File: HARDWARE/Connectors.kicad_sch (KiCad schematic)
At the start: 11 parts, among them J12 Conn_02x08_Odd_Even, J13 Conn_02x10_Odd_Even, J14 Conn_02x15_Odd_Even, J15 Conn_02x17_Odd_Even, J16 Conn_02x36_Odd_Even, J17 Conn_02x36_Odd_Even

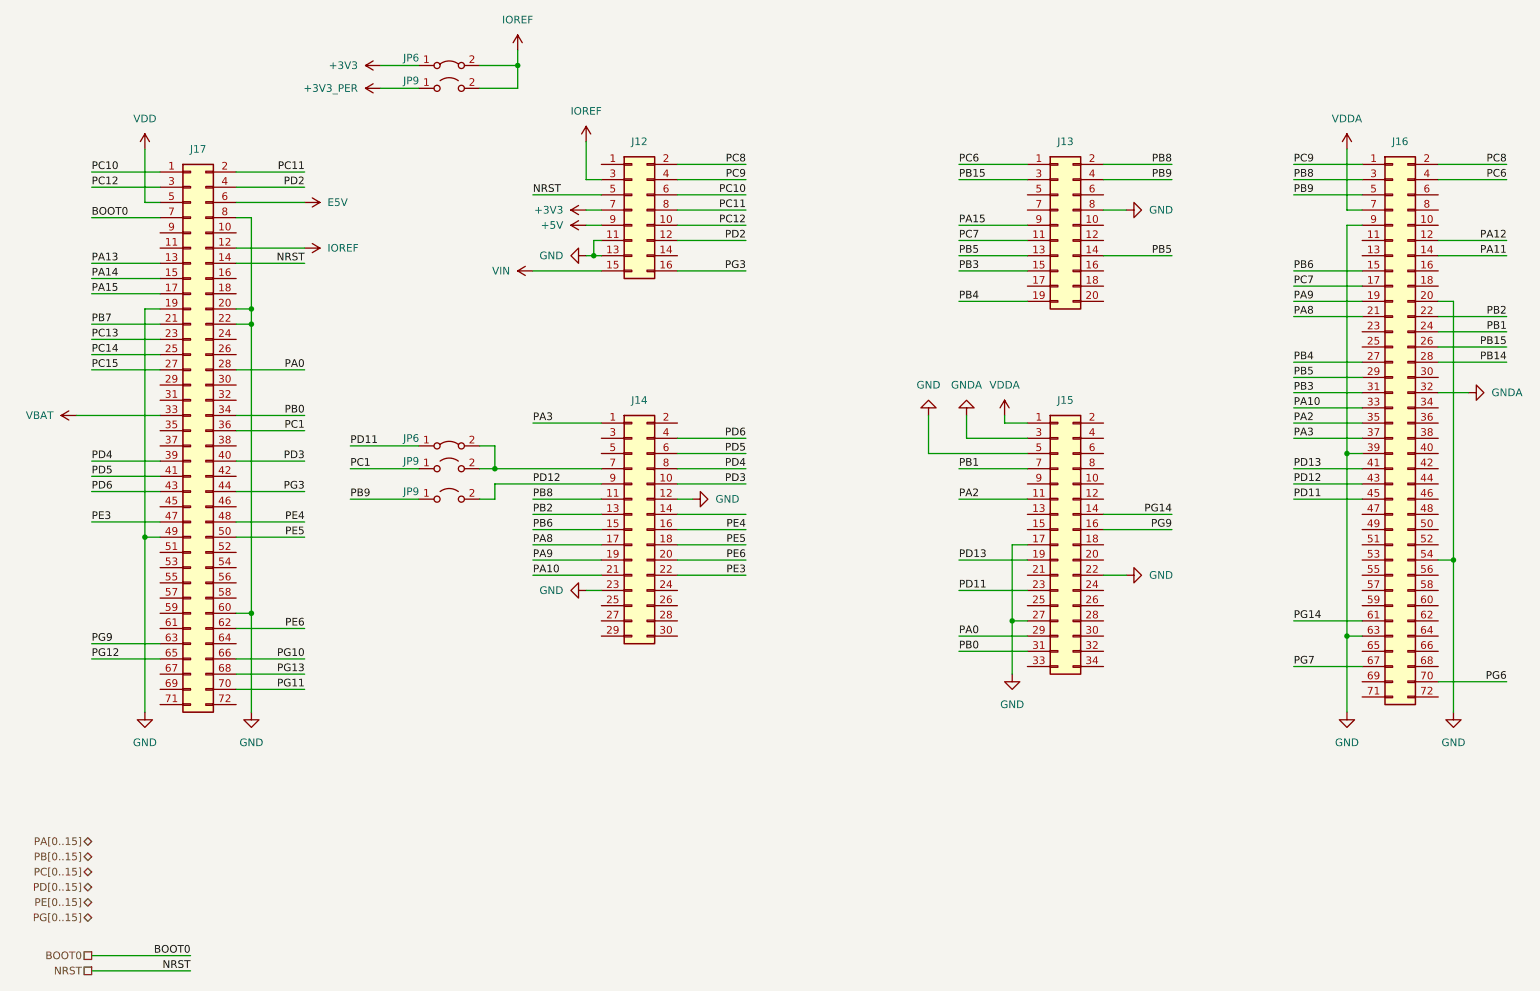
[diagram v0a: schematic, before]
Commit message: schematic capture
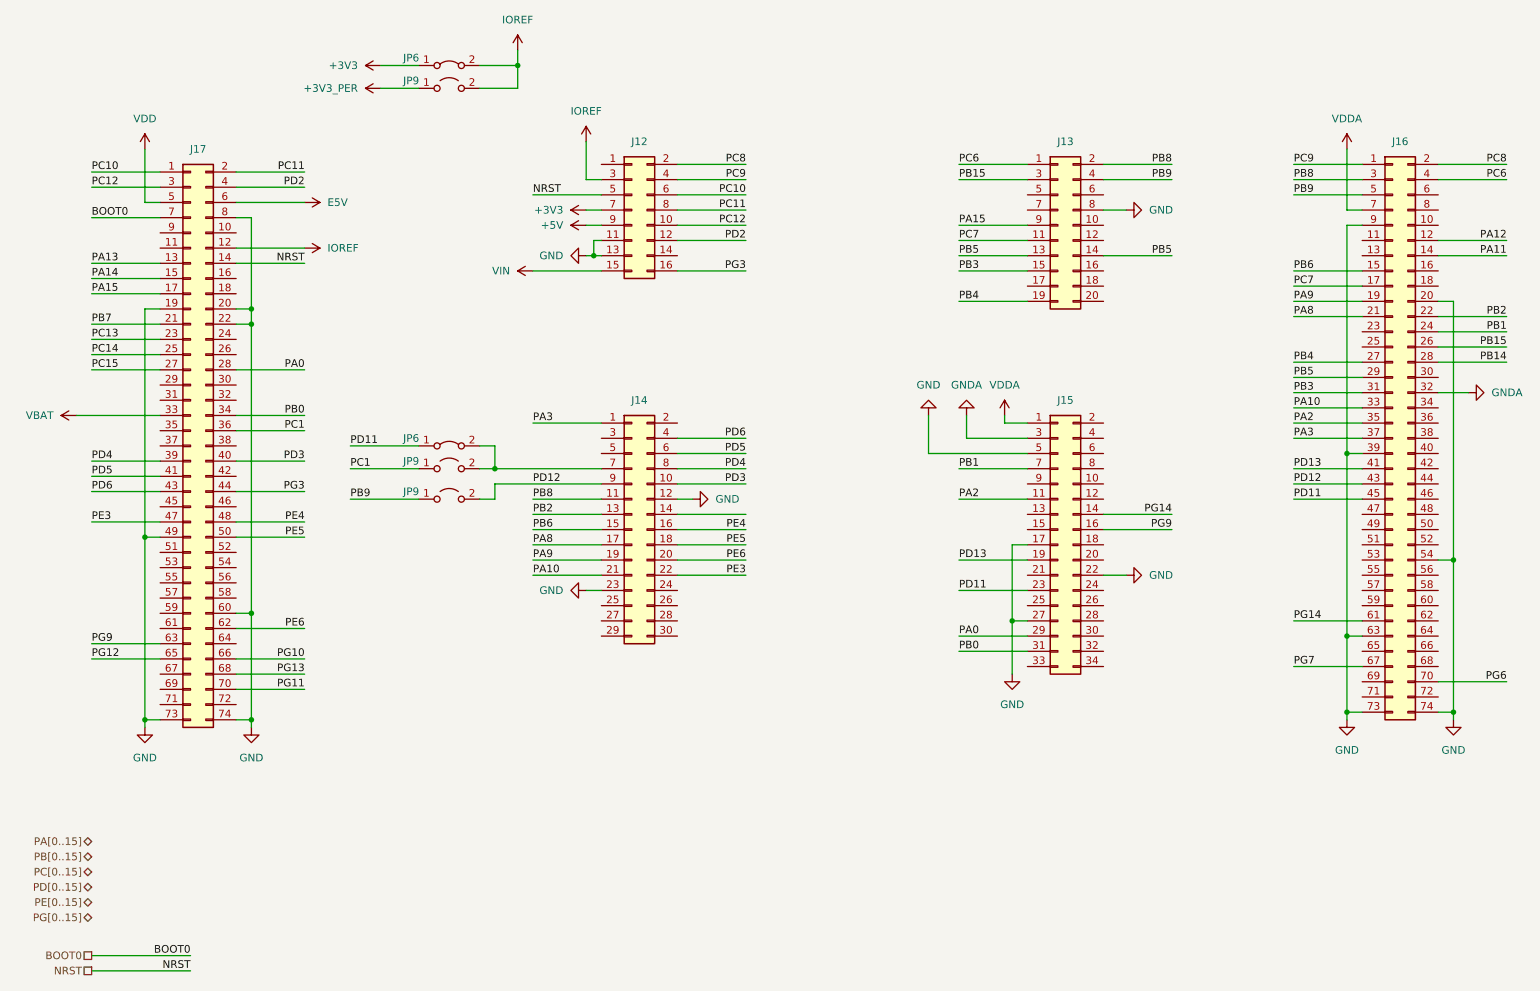
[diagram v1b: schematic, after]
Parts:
- removed J16, J17: Conn_02x36_Odd_Even, symbol Connector_Generic:Conn_02x36_Odd_Even
- added J16, J17: Conn_02x37_Odd_Even, Connector_PinHeader_2.54mm:PinHeader_2x37_P2.54mm_Vertical, symbol Connector_Generic:Conn_02x37_Odd_Even
- J12: footprint (none) -> Connector_PinHeader_2.54mm:PinHeader_2x08_P2.54mm_Vertical
- J13: footprint (none) -> Connector_PinHeader_2.54mm:PinHeader_2x10_P2.54mm_Vertical
- J14: footprint (none) -> Connector_PinHeader_2.54mm:PinHeader_2x15_P2.54mm_Vertical
- J15: footprint (none) -> Connector_PinHeader_2.54mm:PinHeader_2x16_P2.54mm_Vertical
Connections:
- net +5V0: now also J17.6 (Pin_6)
- net BOOT0: now also J17.7 (Pin_7)
- net GND: now also J16.20 (Pin_20), J16.39 (Pin_39), J16.54 (Pin_54), J16.63 (Pin_63), J16.73 (Pin_73), J16.74 (Pin_74), J16.9 (Pin_9), J17.19 (Pin_19), J17.20 (Pin_20), J17.22 (Pin_22), J17.49 (Pin_49), J17.60 (Pin_60), J17.73 (Pin_73), J17.74 (Pin_74), J17.8 (Pin_8)
- net GNDA: now also J16.32 (Pin_32)
- net IOREF: now also J17.12 (Pin_12)
- net NRST: now also J17.14 (Pin_14)
- net PA0: now also J17.28 (Pin_28)
- net PA10: now also J16.33 (Pin_33)
- net PA11: now also J16.14 (Pin_14)
- net PA12: now also J16.12 (Pin_12)
- net PA13: now also J17.13 (Pin_13)
- net PA14: now also J17.15 (Pin_15)
- net PA15: now also J17.17 (Pin_17)
- net PA2: now also J16.35 (Pin_35)
- net PA3: now also J16.37 (Pin_37)
- net PA8: now also J16.21 (Pin_21)
- net PA9: now also J16.19 (Pin_19)
- net PB0: now also J17.34 (Pin_34)
- net PB1: now also J16.24 (Pin_24)
- net PB14: now also J16.28 (Pin_28)
- net PB15: now also J16.26 (Pin_26)
- net PB2: now also J16.22 (Pin_22)
- net PB3: now also J16.31 (Pin_31)
- net PB4: now also J16.27 (Pin_27)
- net PB5: now also J16.29 (Pin_29)
- net PB6: now also J16.15 (Pin_15)
- net PB7: now also J17.21 (Pin_21)
- net PB8: now also J16.3 (Pin_3)
- net PB9: now also J16.5 (Pin_5)
- net PC1: now also J17.36 (Pin_36)
- net PC10: now also J17.1 (Pin_1)
- net PC11: now also J17.2 (Pin_2)
- net PC12: now also J17.3 (Pin_3)
- net PC13: now also J17.23 (Pin_23)
- net PC14: now also J17.25 (Pin_25)
- net PC15: now also J17.27 (Pin_27)
- net PC6: now also J16.4 (Pin_4)
- net PC7: now also J16.17 (Pin_17)
- net PC8: now also J16.2 (Pin_2)
- net PC9: now also J16.1 (Pin_1)
- net PD11: now also J16.45 (Pin_45)
- net PD12: now also J16.43 (Pin_43)
- net PD13: now also J16.41 (Pin_41)
- net PD2: now also J17.4 (Pin_4)
- net PD3: now also J17.40 (Pin_40)
- net PD4: now also J17.39 (Pin_39)
- net PD5: now also J17.41 (Pin_41)
- net PD6: now also J17.43 (Pin_43)
- net PE3: now also J17.47 (Pin_47)
- net PE4: now also J17.48 (Pin_48)
- net PE5: now also J17.50 (Pin_50)
- net PE6: now also J17.62 (Pin_62)
- net PG10: now also J17.66 (Pin_66)
- net PG11: now also J17.70 (Pin_70)
- net PG12: now also J17.65 (Pin_65)
- net PG13: now also J17.68 (Pin_68)
- net PG14: now also J16.61 (Pin_61)
- net PG3: now also J17.44 (Pin_44)
- net PG6: now also J16.70 (Pin_70)
- net PG7: now also J16.67 (Pin_67)
- net PG9: now also J17.63 (Pin_63)
- net VBAT: now also J17.33 (Pin_33)
- net VDD: now also J17.5 (Pin_5)
- net VDDA: now also J16.7 (Pin_7)
